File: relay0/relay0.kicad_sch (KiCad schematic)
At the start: 15 parts, among them J1 2601-1106, J2 2601-1106, J3 2601-1102, K1 J107F1AS2012VDC.80, K2 J107F1AS2012VDC.80, K3 J107F1AS2012VDC.80, K4 J107F1AS2012VDC.80, K5 J107F1AS2012VDC.80, K6 J107F1AS2012VDC.80

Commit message: Readme updates
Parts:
- J1, J2: footprint footprints:CONN6_2601-1106_WAG -> 2601_1106:CONN6_2601-1106_WAG
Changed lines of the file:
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@@
 			)
 		)
-		(property "Footprint" "footprints:CONN6_2601-1106_WAG"
+		(property "Footprint" "2601_1106:CONN6_2601-1106_WAG"
 			(at 40.64 55.88 0)
 			(effects
@@
 			)
 		)
-		(property "Footprint" "footprints:CONN6_2601-1106_WAG"
+		(property "Footprint" "2601_1106:CONN6_2601-1106_WAG"
 			(at 156.21 59.69 0)
 			(effects

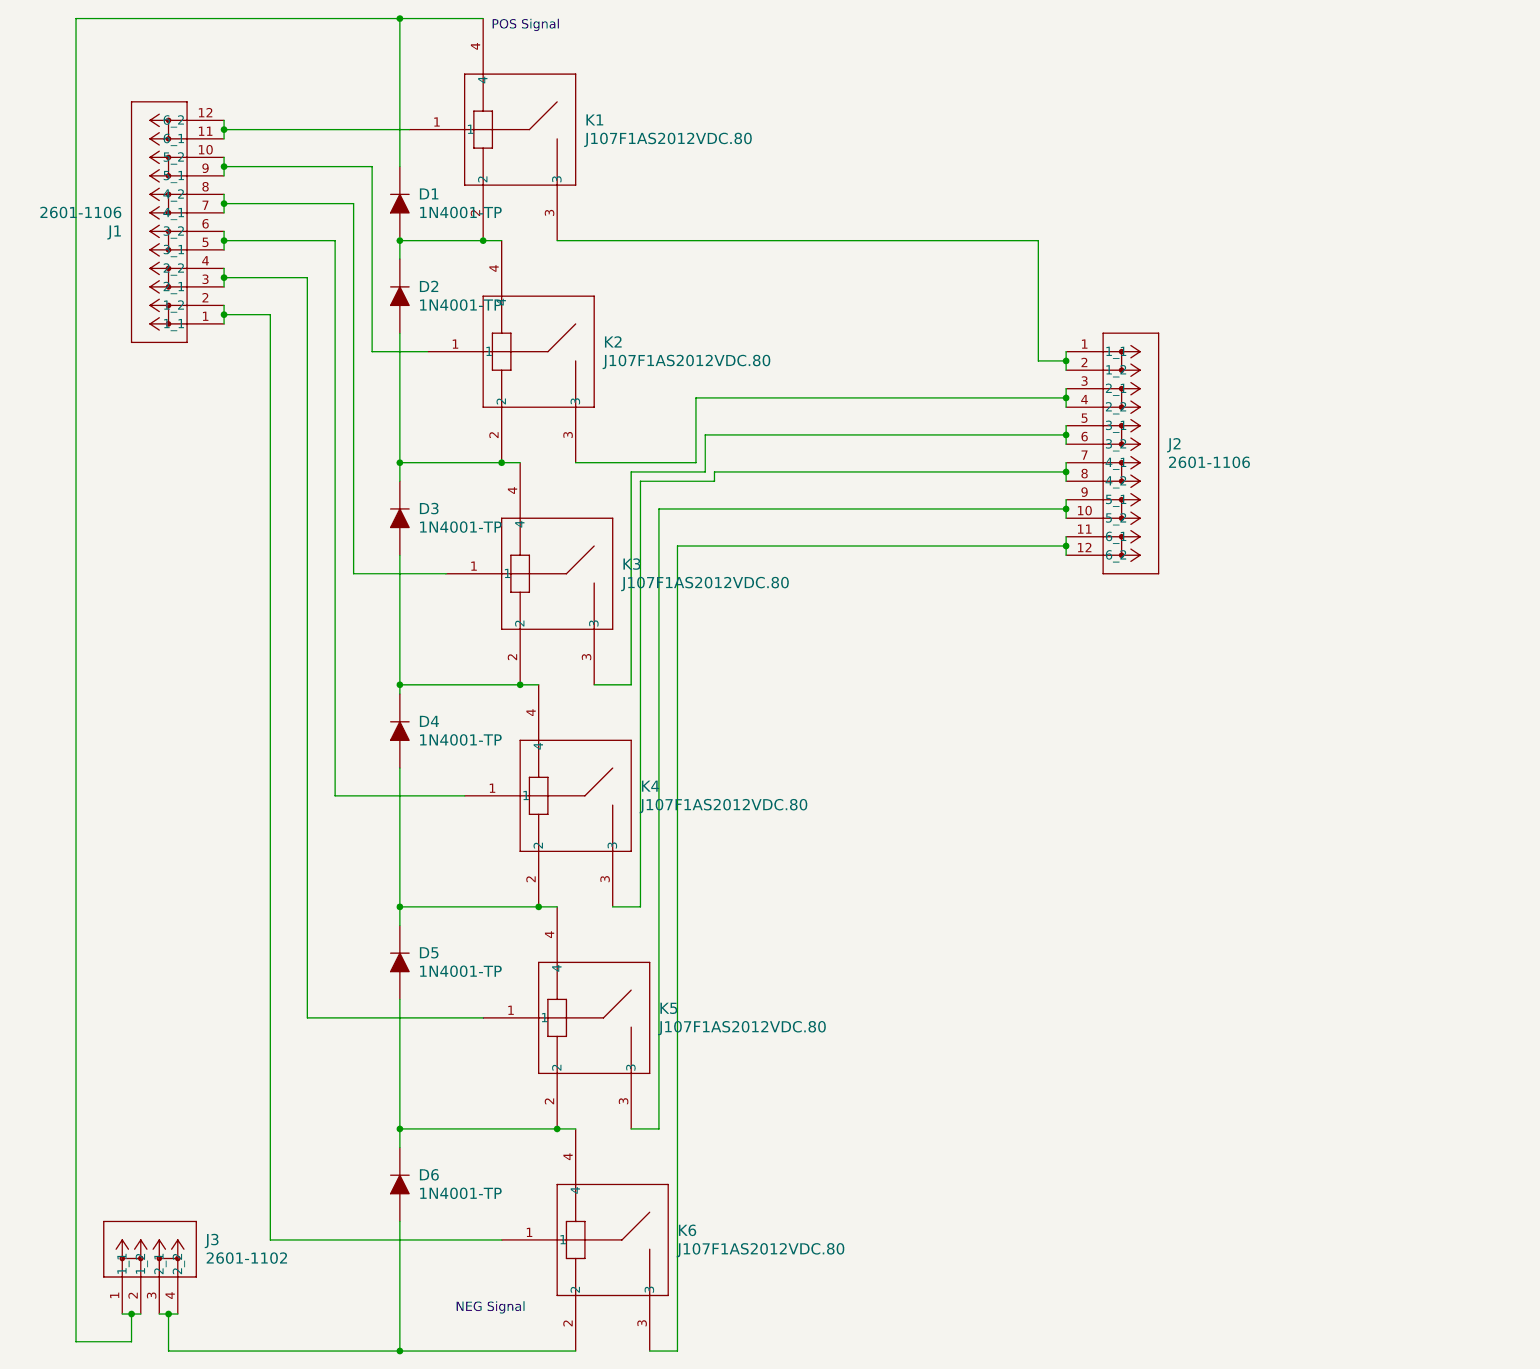
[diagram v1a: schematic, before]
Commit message: PCB Design updates
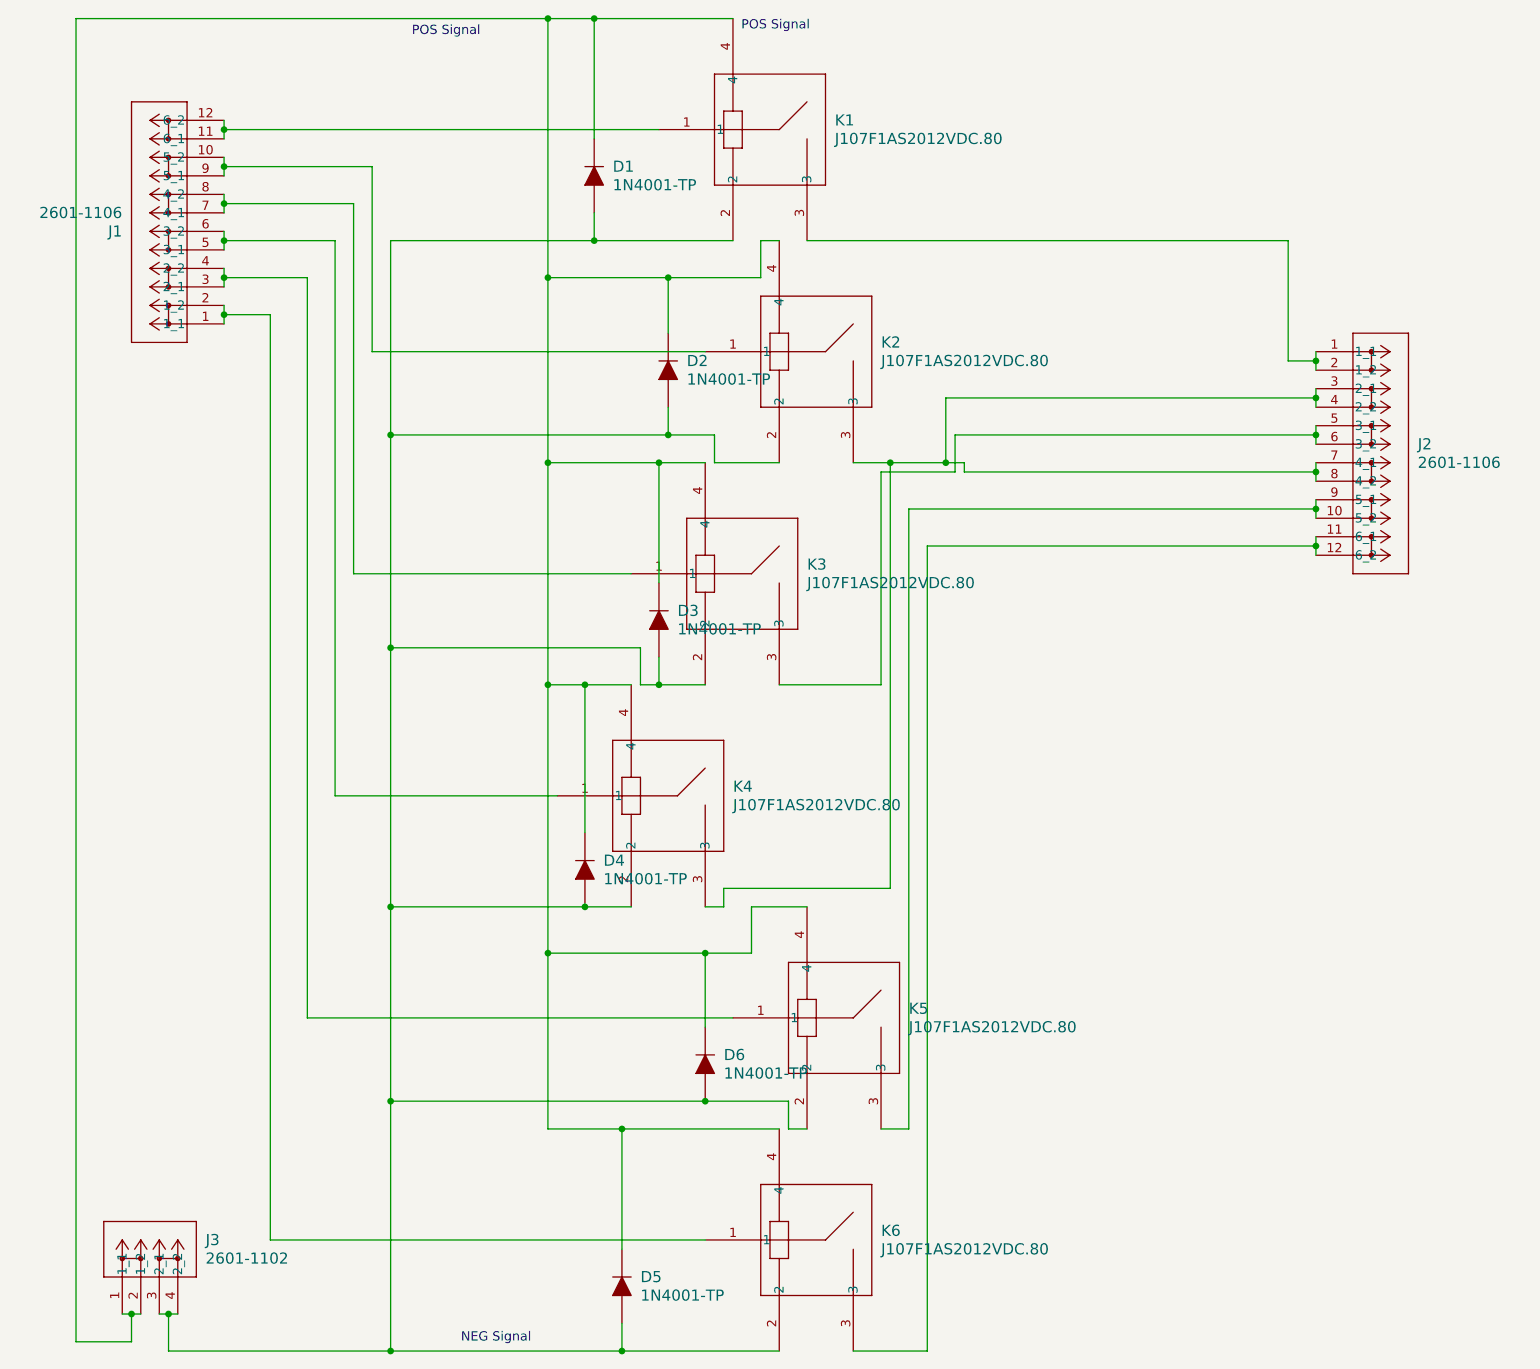
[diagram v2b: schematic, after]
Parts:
- removed D1, D5: 1N4001-TP, digikey-footprints:DO-41, symbol dk_Diodes-Rectifiers-Single:1N4001-TP
- added D3, D6: 1N4001-TP, digikey-footprints:DO-41, symbol dk_Diodes-Rectifiers-Single:1N4001-TP
- renumbered D3 to D1, D6 to D5
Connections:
- net at D2.A, K2.2: now also D1.A, D4.A, D5.A, J3.3 (2_1), J3.4 (2_2), K1.2, K3.2, K4.2, K5.2, K6.2, D3.A, D6.A; no longer D1.K, K3.4
- net at D2.K, K2.4: now also D1.K, D4.K, D5.K, J3.1 (1_1), J3.2 (1_2), K1.4, K3.4, K4.4, K5.4, K6.4, D3.K, D6.K; no longer K1.2
- net at J2.3 (2_1), J2.4 (2_2), K2.3: now also J2.7 (4_1), J2.8 (4_2), K4.3
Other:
- moved on the sheet: D1, D5, J2, K1, K2, K3, K4, K5, K6
